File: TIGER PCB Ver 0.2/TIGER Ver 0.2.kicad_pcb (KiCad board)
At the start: 2 copper layers, 68.5 x 58.2 mm, 52 parts, among them J1 USB4105-GF-A, J10 Conn_01x09_Socket, J11 Conn_01x09_Socket, J2 Servo 1, J3 Servo 3, J4 Servo 2, J5 Servo 4, J6 Battery Connector, J9 MSD-4-A, SW1 SW_RESET, SW2 SW_RESET, U1 AMS1117-3.3, U2 ESP32-S3-WROOM-1, U3 AMS1117-5.0, U4 MPL3115A2, U5 BMI270

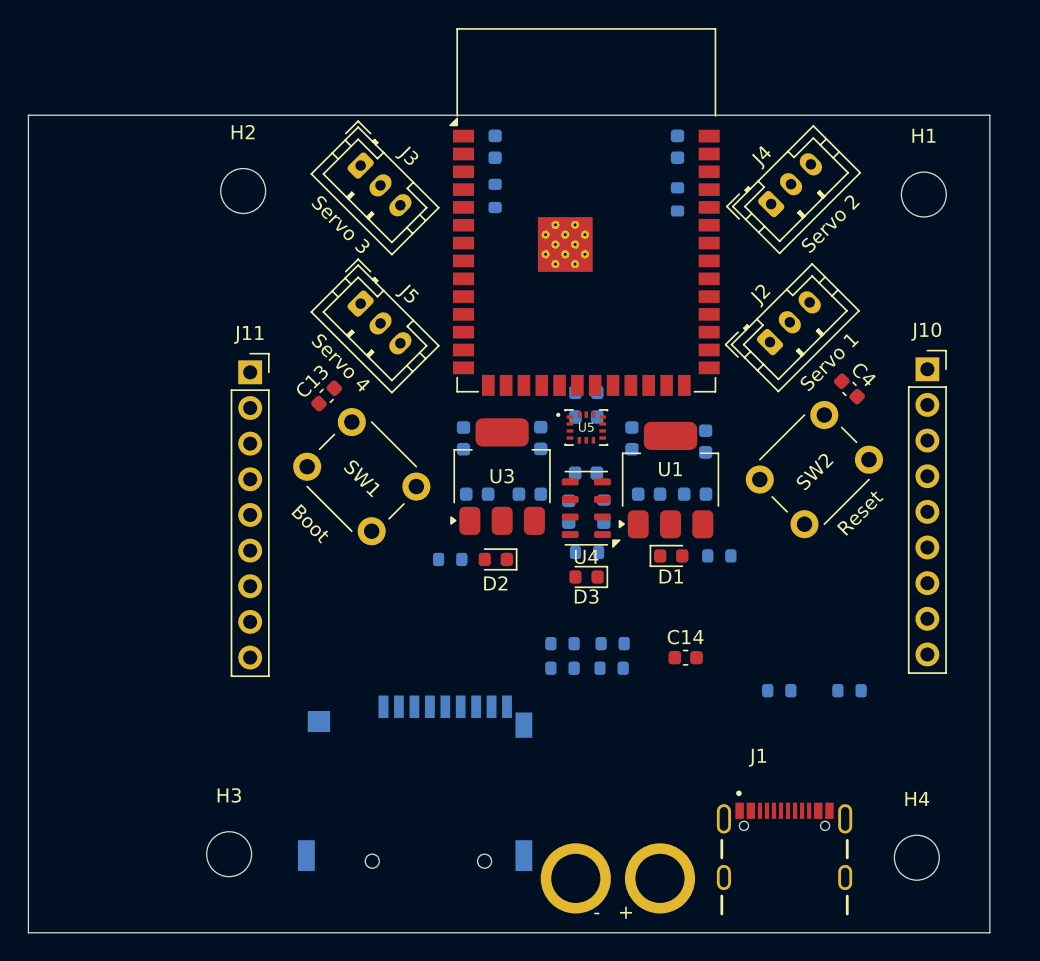
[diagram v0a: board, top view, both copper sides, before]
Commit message: Finished Layout
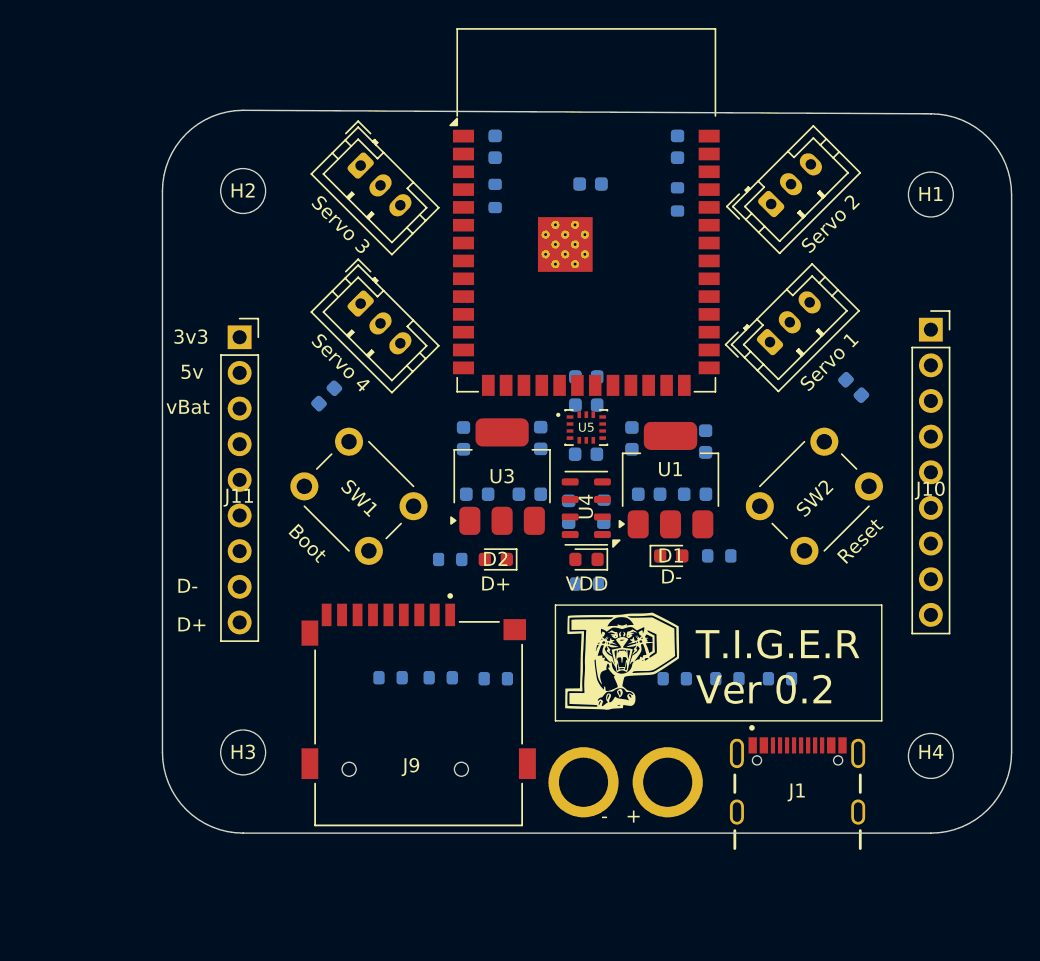
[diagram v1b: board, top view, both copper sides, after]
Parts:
- added G***: LOGO, .Custom Footprints:PHS Tigers Logo, F.Cu at (142.9, 105.3)
- C13, C14, C4: moved to B.Cu
- J9: moved to F.Cu
- moved C4 23.5 mm to (140.0, 71.2), turned to 0 degrees
- moved C14 22.7 mm to (158.8, 85.8), turned to 135 degrees
- moved R11 12.5 mm to (129.3, 106.4)
- moved R9 12.5 mm to (125.8, 106.4)
- moved R10 8.28 mm to (133.2, 106.5), turned to 180 degrees
- moved R12 8.04 mm to (146.0, 106.5), turned to 0 degrees
- moved H3 7.32 mm to (115.2, 111.8)
- moved H4 7.32 mm to (164.2, 112.0)
- moved J6 6.87 mm to (142.5, 118.4)
- moved J9 6.55 mm to (127.8, 109.7), turned to 0 degrees
- moved R4 5.02 mm to (153.5, 106.5)
- moved J1 4.75 mm to (154.8, 116.0)
- moved R3 3.80 mm to (149.8, 106.5)
- moved J10 2.83 mm to (164.2, 81.6)
- moved J11 2.61 mm to (115.0, 82.2)
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- renumbered D3 to VDD
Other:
- board size 68.5 x 58.2 mm -> 60.5 x 51.5 mm
- board text added: "3v3"
- board text added: "5v"
- board text added: "D+"
- board text added: "D-"
- board text added: "T.I.G.E.R Ver 0.2"
- board text added: "vBat"
